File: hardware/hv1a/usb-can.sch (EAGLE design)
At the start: 5 parts, among them U1 CP2130, U2 MCP2515-ML, U3 MCP2561, U4 MCP1700-330

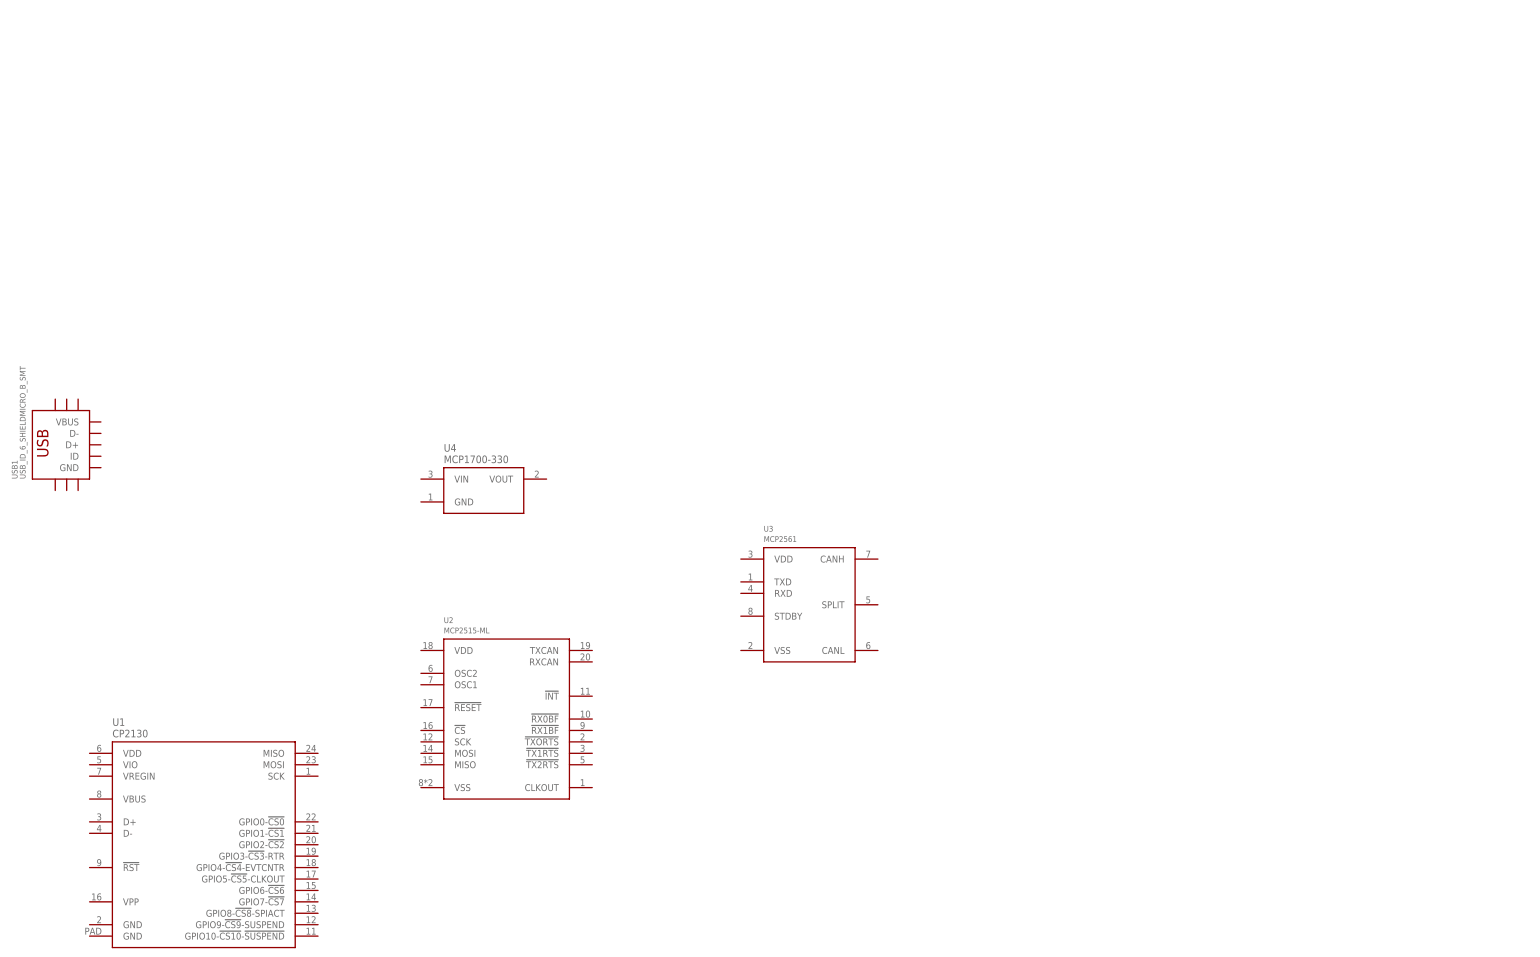
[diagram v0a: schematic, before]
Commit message: Work
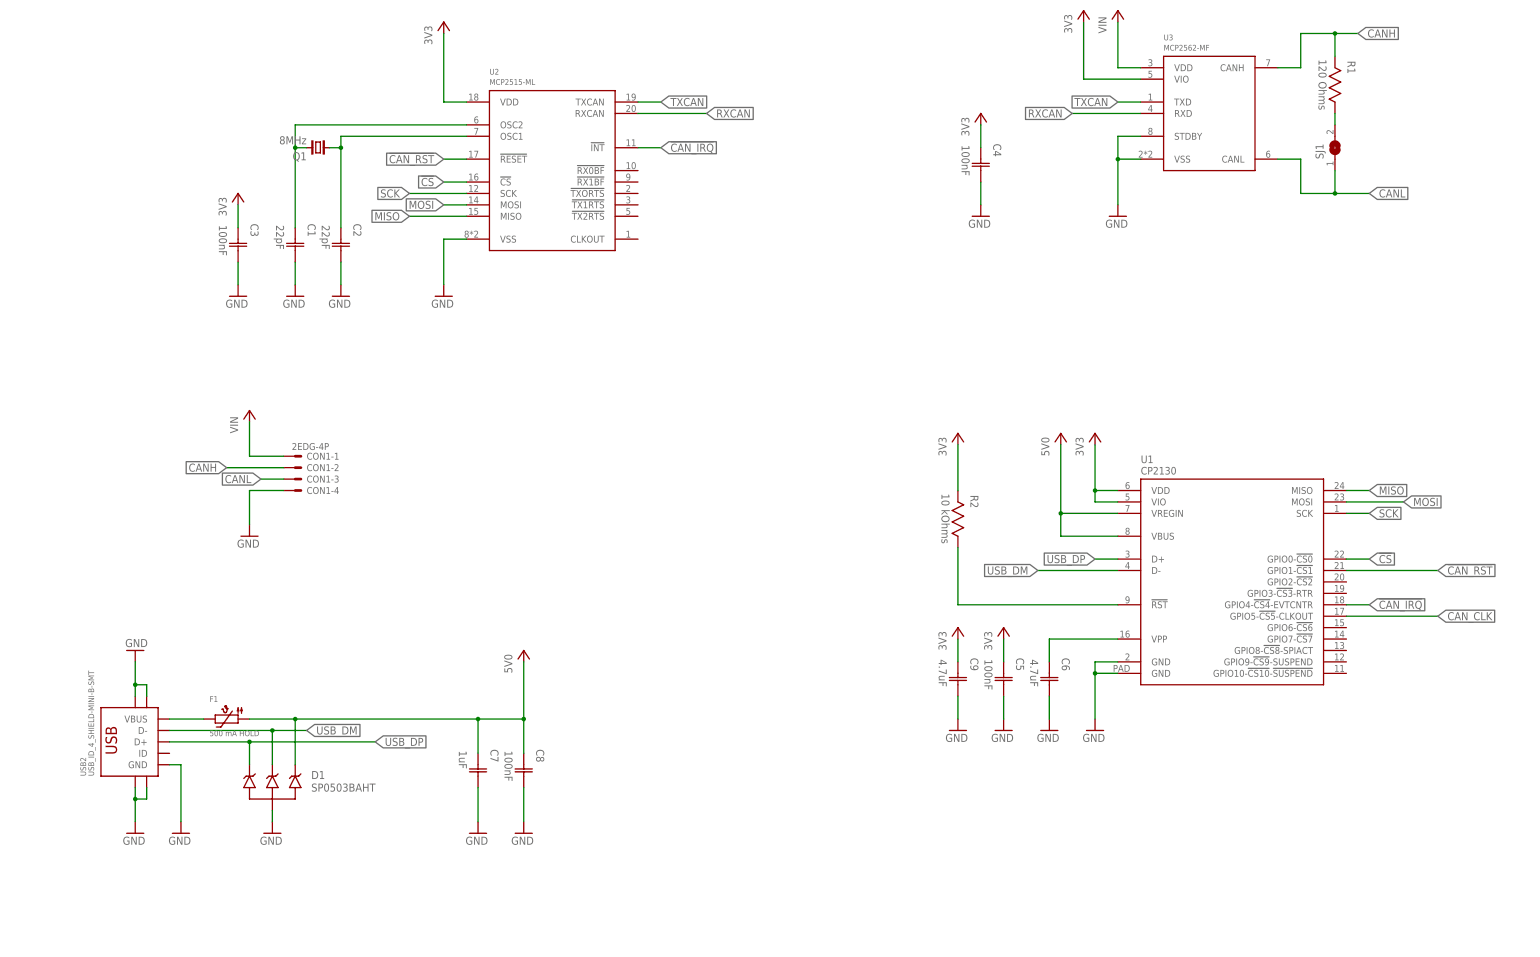
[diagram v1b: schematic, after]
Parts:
- removed U4: MCP1700-330, Microchip:MCP1700-330
- removed USB1: USB_ID_6_SHIELDMICRO_B_SMT, USB Connector:USB_ID_6_SHIELDMICRO_B_SMT
- added C1, C2: 22pF, Capacitor:CAPACITOR-0603
- added C3, C4, C5, C8: 100nF, Capacitor:CAPACITOR-0603
- added C6, C9: 4.7uF, Capacitor:CAPACITOR-0603
- added C7: 1uF, Capacitor:CAPACITOR-0603
- added CON1: 2EDG-4P, Generic Connector:2EDG-4P
- added D1: SP0503BAHT, TVS:SP0503BAHT
- added F1: 500 mA HOLD, PTC Fuses:PTC1206
- added Q1: 8MHz, Crystal:CRYSTAL2-SMD-5X3
- added R1: 120 Ohms, Resistor:RESISTOR-0603
- added R2: 10 kOhms, Resistor:RESISTOR-0603
- added SJ1: (no value), Solder Jumper:SJS
- added USB2: USB_ID_4_SHIELD-MINI-B-SMT, USB Connector:USB_ID_4_SHIELD-MINI-B-SMT
- U3: value MCP2561 -> MCP2562-MF; device Microchip:MCP2561 -> Microchip:MCP2562-MF
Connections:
- new net !CAN_IRQ: U1.GPIO4-!CS4!-EVTCNTR, U2.!INT!
- new net !CAN_RST: U1.GPIO1-!CS1, U2.!RESET!
- new net !CS: U1.GPIO0-!CS0, U2.!CS!
- new net 3V3: C3.C1, C4.C1, C5.C1, C9.C1, R2.2, U1.VDD, U1.VIO, U2.VDD, U3.VIO
- new net 5V0: C7.C1, C8.C1, D1.4, F1.1, U1.VBUS, U1.VREGIN
- new net CANH: CON1-2.S, R1.2, U3.CANH
- new net CANL: CON1-3.S, SJ1.1, U3.CANL
- new net CAN_CLK: U1.GPIO5-!CS5!-CLKOUT
- new net GND: C1.C2, C2.C2, C3.C2, C4.C2, C5.C2, C6.C2, C7.C2, C8.C2, C9.C2, CON1-4.S, D1.1, U1.GND@0, U1.GND@1, U2.VSS, U3.STDBY, U3.VSS, USB2.GND, USB2.SHIELD@0, USB2.SHIELD@1, USB2.SHIELD@2, USB2.SHIELD@3
- new net MISO: U1.MISO, U2.MISO
- new net MOSI: U1.MOSI, U2.MOSI
- new net N$1: C2.C1, Q1.1, U2.OSC1
- new net N$2: C1.C1, Q1.2, U2.OSC2
- new net N$3: R1.1, SJ1.2
- new net N$4: C6.C1, U1.VPP
- new net N$5: R2.1, U1.!RST
- new net N$6: F1.2, USB2.VBUS
- new net RXCAN: U2.RXCAN, U3.RXD
- new net SCK: U1.SCK, U2.SCK
- new net TXCAN: U2.TXCAN, U3.TXD
- new net USB_DM: D1.3, U1.D-, USB2.D-
- new net USB_DP: D1.2, U1.D+, USB2.D+
- new net VIN: CON1-1.S, U3.VDD
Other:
- moved on the sheet: U1, U2, U3
